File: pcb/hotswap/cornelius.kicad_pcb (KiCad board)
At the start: 2 copper layers, 271.8 x 128.2 mm, 126 parts, among them J1 AVR-ISP-6, SW1 SW_Push, U1 ATmega32U4-M, U2 PRTR5V0U2X, Y1 16MHz

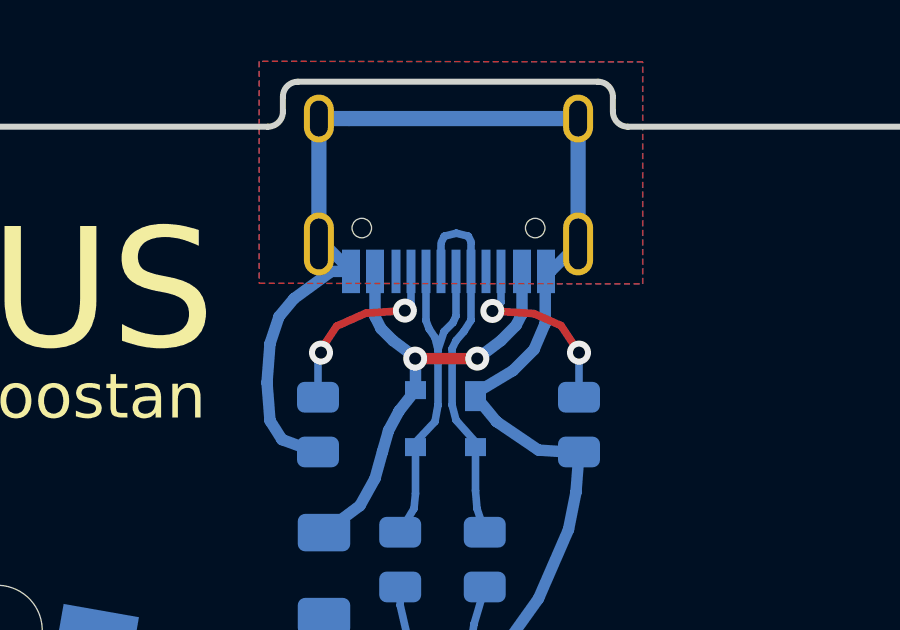
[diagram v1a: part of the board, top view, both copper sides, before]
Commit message: Update solder pcb
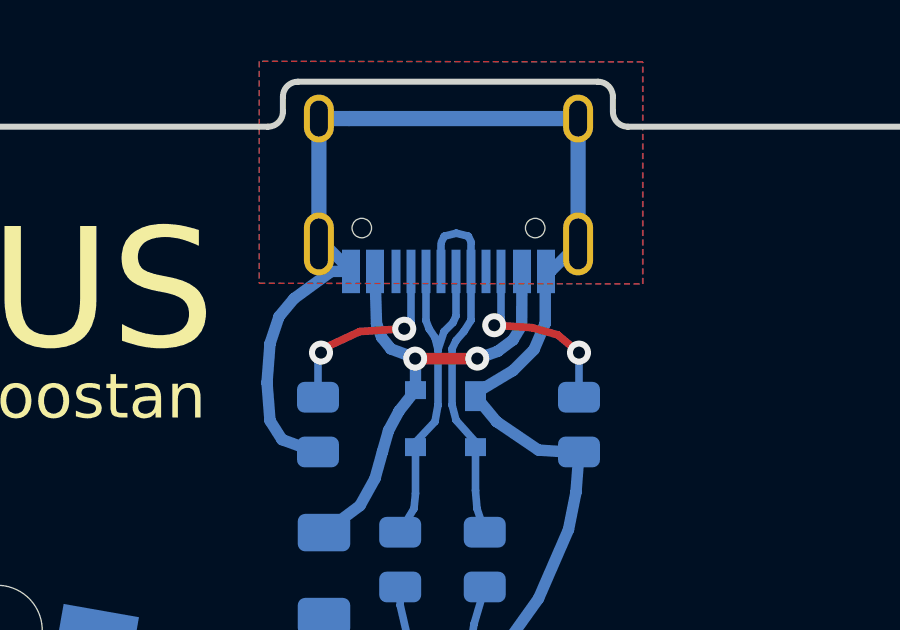
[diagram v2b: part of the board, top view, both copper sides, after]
